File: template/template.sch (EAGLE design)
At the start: 36 parts, among them CN1 8P8C-LED, SW1 SWITCH_TACTILETOP, U1 STM32F103C8, U2 NCV7351D1E, U3 AP65111AWU-7, X1 CSTCE8M00G55

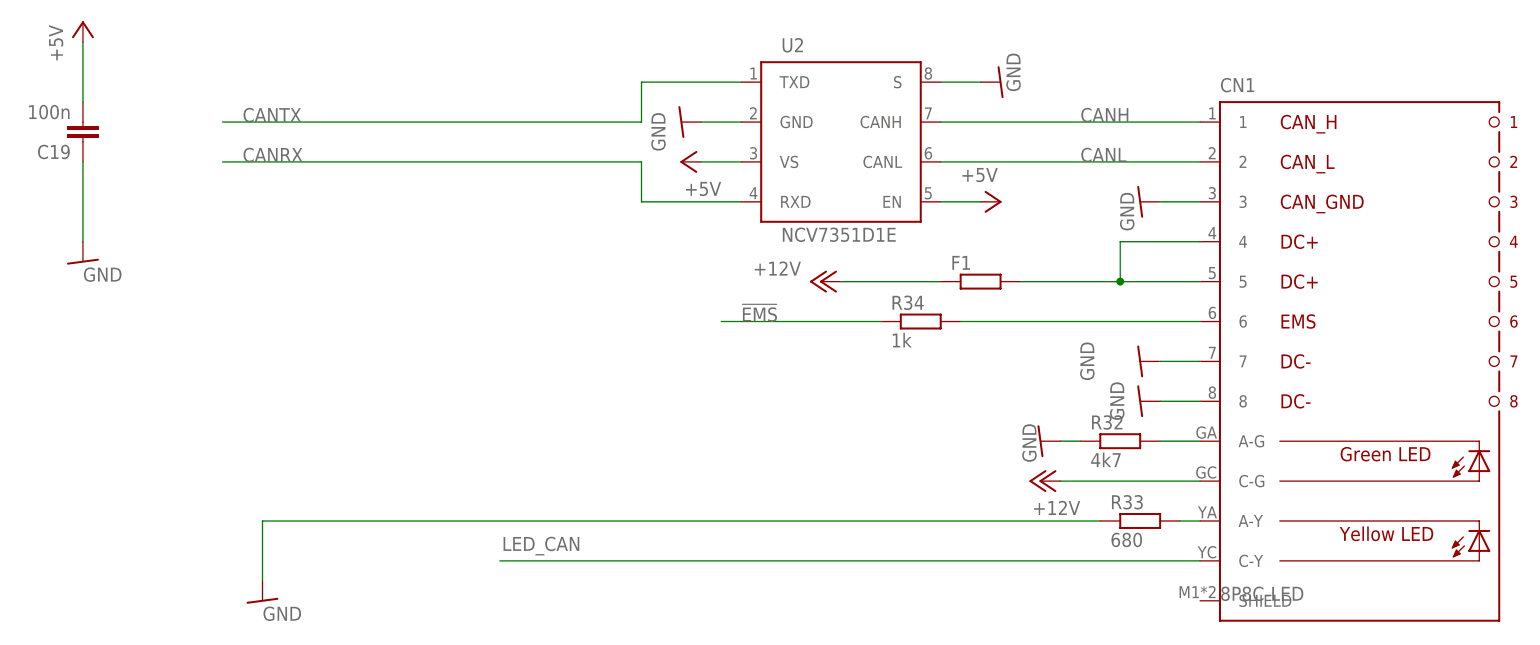
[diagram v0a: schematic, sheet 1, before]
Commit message: テンプレートのライブラリの更新
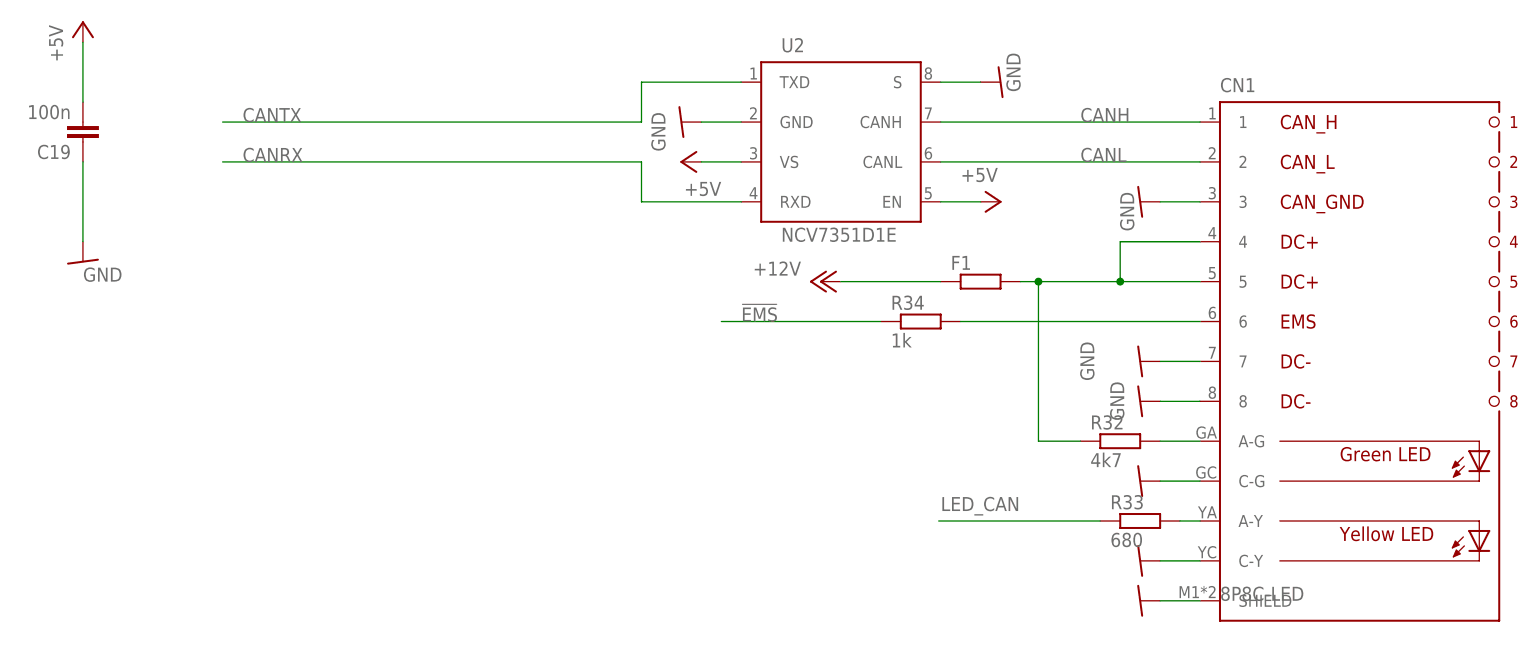
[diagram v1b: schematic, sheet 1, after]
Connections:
- net +24V: no longer CN1.C-G
- net GND: no longer R32.1, R33.1
- net GNDIO: now also CN1.C-G, CN1.C-Y, CN1.SHIELD
- net LED_CAN: now also R33.1; no longer CN1.C-Y
- net N$36: now also R32.1
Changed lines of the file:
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@@
 <?xml version="1.0" encoding="utf-8"?>
 <!DOCTYPE eagle SYSTEM "eagle.dtd">
-<eagle version="9.3.2">
+<eagle version="9.4.2">
 <drawing>
 <settings>
@@
 <part name="P+28" library="supply1" library_urn="urn:adsk.eagle:library:371" deviceset="+5V" device=""/>
 <part name="12V" library="supply1" library_urn="urn:adsk.eagle:library:371" deviceset="+12V" device=""/>
-<part name="P+30" library="supply1" library_urn="urn:adsk.eagle:library:371" deviceset="+12V" device=""/>
 <part name="U1" library="stm32_mcu" deviceset="STM32F103C8" device=""/>
 <part name="P+32" library="supply1" library_urn="urn:adsk.eagle:library:371" deviceset="+3V3" device=""/>
@@
 <part name="+3V1" library="supply1" library_urn="urn:adsk.eagle:library:371" deviceset="+3V3" device=""/>
 <part name="R4" library="rcl" library_urn="urn:adsk.eagle:library:334" deviceset="R-US_" device="R0603" package3d_urn="urn:adsk.eagle:package:23555/3" value="47k"/>
+<part name="GND9" library="supply1" library_urn="urn:adsk.eagle:library:371" deviceset="GNDIO" device=""/>
 </parts>
 <sheets>
@@
 <instance part="GND18" gate="G$1" x="127" y="77.47" smashed="yes" rot="R90"/>
 <instance part="GND19" gate="G$1" x="144.78" y="62.23" smashed="yes" rot="R270"/>
-<instance part="GND20" gate="G$1" x="132.08" y="31.75" smashed="yes" rot="R270"/>
+<instance part="GND20" gate="G$1" x="144.78" y="26.67" smashed="yes" rot="R270"/>
 <instance part="GND21" gate="G$1" x="144.78" y="41.91" smashed="yes" rot="R270"/>
-<instance part="GND22" gate="G$1" x="33.02" y="11.43" smashed="yes"/>
+<instance part="GND22" gate="G$1" x="144.78" y="16.51" smashed="yes" rot="R270"/>
 <instance part="F1" gate="G$1" x="124.46" y="52.07" smashed="yes">
 <attribute name="NAME" x="120.65" y="53.5686" size="1.778" layer="95"/>
@@
 <attribute name="VALUE" x="101.6" y="54.61" size="1.778" layer="96" rot="R180"/>
 </instance>
-<instance part="P+30" gate="1" x="132.08" y="26.67" smashed="yes" rot="R90">
-<attribute name="VALUE" x="137.16" y="24.13" size="1.778" layer="96" rot="R180"/>
-</instance>
+<instance part="GND9" gate="G$1" x="144.78" y="11.43" smashed="yes" rot="R270"/>
 </instances>
 <busses>
@@
 <wire x1="152.4" y1="52.07" x2="142.24" y2="52.07" width="0.1524" layer="91"/>
 <pinref part="CN1" gate="G$1" pin="4"/>
-<wire x1="142.24" y1="52.07" x2="129.54" y2="52.07" width="0.1524" layer="91"/>
+<wire x1="142.24" y1="52.07" x2="131.826" y2="52.07" width="0.1524" layer="91"/>
+<wire x1="131.826" y1="52.07" x2="129.54" y2="52.07" width="0.1524" layer="91"/>
 <wire x1="152.4" y1="57.15" x2="142.24" y2="57.15" width="0.1524" layer="91"/>
 <wire x1="142.24" y1="57.15" x2="142.24" y2="52.07" width="0.1524" layer="91"/>
 <junction x="142.24" y="52.07"/>
+<pinref part="R32" gate="G$1" pin="1"/>
+<wire x1="137.16" y1="31.75" x2="131.826" y2="31.75" width="0.1524" layer="91"/>
+<wire x1="131.826" y1="31.75" x2="131.826" y2="52.07" width="0.1524" layer="91"/>
+<junction x="131.826" y="52.07"/>
 </segment>
 </net>
@@
 <pinref part="12V" gate="1" pin="+12V"/>
 </segment>
-<segment>
-<pinref part="P+30" gate="1" pin="+12V"/>
-<pinref part="CN1" gate="G$1" pin="C-G"/>
-<wire x1="134.62" y1="26.67" x2="152.4" y2="26.67" width="0.1524" layer="91"/>
-</segment>
 </net>
 <net name="GND" class="0">
-<segment>
-<pinref part="R33" gate="G$1" pin="1"/>
-<wire x1="33.02" y1="21.59" x2="139.7" y2="21.59" width="0.1524" layer="91"/>
-<wire x1="33.02" y1="21.59" x2="33.02" y2="13.97" width="0.1524" layer="91"/>
-<pinref part="GND22" gate="G$1" pin="GNDIO"/>
-<label x="33.02" y="8.89" size="1.778" layer="95"/>
-</segment>
 <segment>
 <pinref part="C19" gate="G$1" pin="1"/>
@@
 </segment>
 <segment>
-<pinref part="GND20" gate="G$1" pin="GNDIO"/>
-<pinref part="R32" gate="G$1" pin="1"/>
-<wire x1="134.62" y1="31.75" x2="137.16" y2="31.75" width="0.1524" layer="91"/>
-<label x="129.794" y="34.036" size="1.778" layer="95" rot="R270"/>
-</segment>
-<segment>
 <pinref part="CN1" gate="G$1" pin="8"/>
 <pinref part="GND23" gate="G$1" pin="GNDIO"/>
@@
 </segment>
 </net>
+<net name="GNDIO" class="0">
+<segment>
+<pinref part="CN1" gate="G$1" pin="C-G"/>
+<pinref part="GND20" gate="G$1" pin="GNDIO"/>
+<wire x1="147.32" y1="26.67" x2="152.4" y2="26.67" width="0.1524" layer="91"/>
+</segment>
+<segment>
+<pinref part="CN1" gate="G$1" pin="C-Y"/>
+<pinref part="GND22" gate="G$1" pin="GNDIO"/>
+<wire x1="147.32" y1="16.51" x2="152.4" y2="16.51" width="0.1524" layer="91"/>
+</segment>
+<segment>
+<pinref part="CN1" gate="G$1" pin="SHIELD"/>
+<pinref part="GND9" gate="G$1" pin="GNDIO"/>
+<wire x1="147.32" y1="11.43" x2="152.4" y2="11.43" width="0.1524" layer="91"/>
+</segment>
+</net>
 <net name="LED_CAN" class="0">
 <segment>
-<pinref part="CN1" gate="G$1" pin="C-Y"/>
-<wire x1="152.4" y1="16.51" x2="63.246" y2="16.51" width="0.1524" layer="91"/>
-<label x="63.5" y="17.78" size="1.778" layer="95"/>
+<pinref part="R33" gate="G$1" pin="1"/>
+<wire x1="139.7" y1="21.59" x2="119.126" y2="21.59" width="0.1524" layer="91"/>
+<label x="119.38" y="22.86" size="1.778" layer="95"/>
 </segment>
 </net>
@@
 packages will not be understood (or retained) with this version.
 </note>
+<note version="8.4" severity="warning">
+Since Version 8.4, EAGLE supports properties for SPICE simulation.
+Probes in schematics and SPICE mapping objects found in parts and library devices
+will not be understood with this version. Update EAGLE to the latest version
+for full support of SPICE simulation.
+</note>
 </compatibility>
